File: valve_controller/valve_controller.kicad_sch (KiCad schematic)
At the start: 12 parts, among them J1 CDM1204-04A-FP-F9-67, U1 OPA197xD, U2 ADS1115IDGS, U3 MCP4728, U4 ESP32-S3

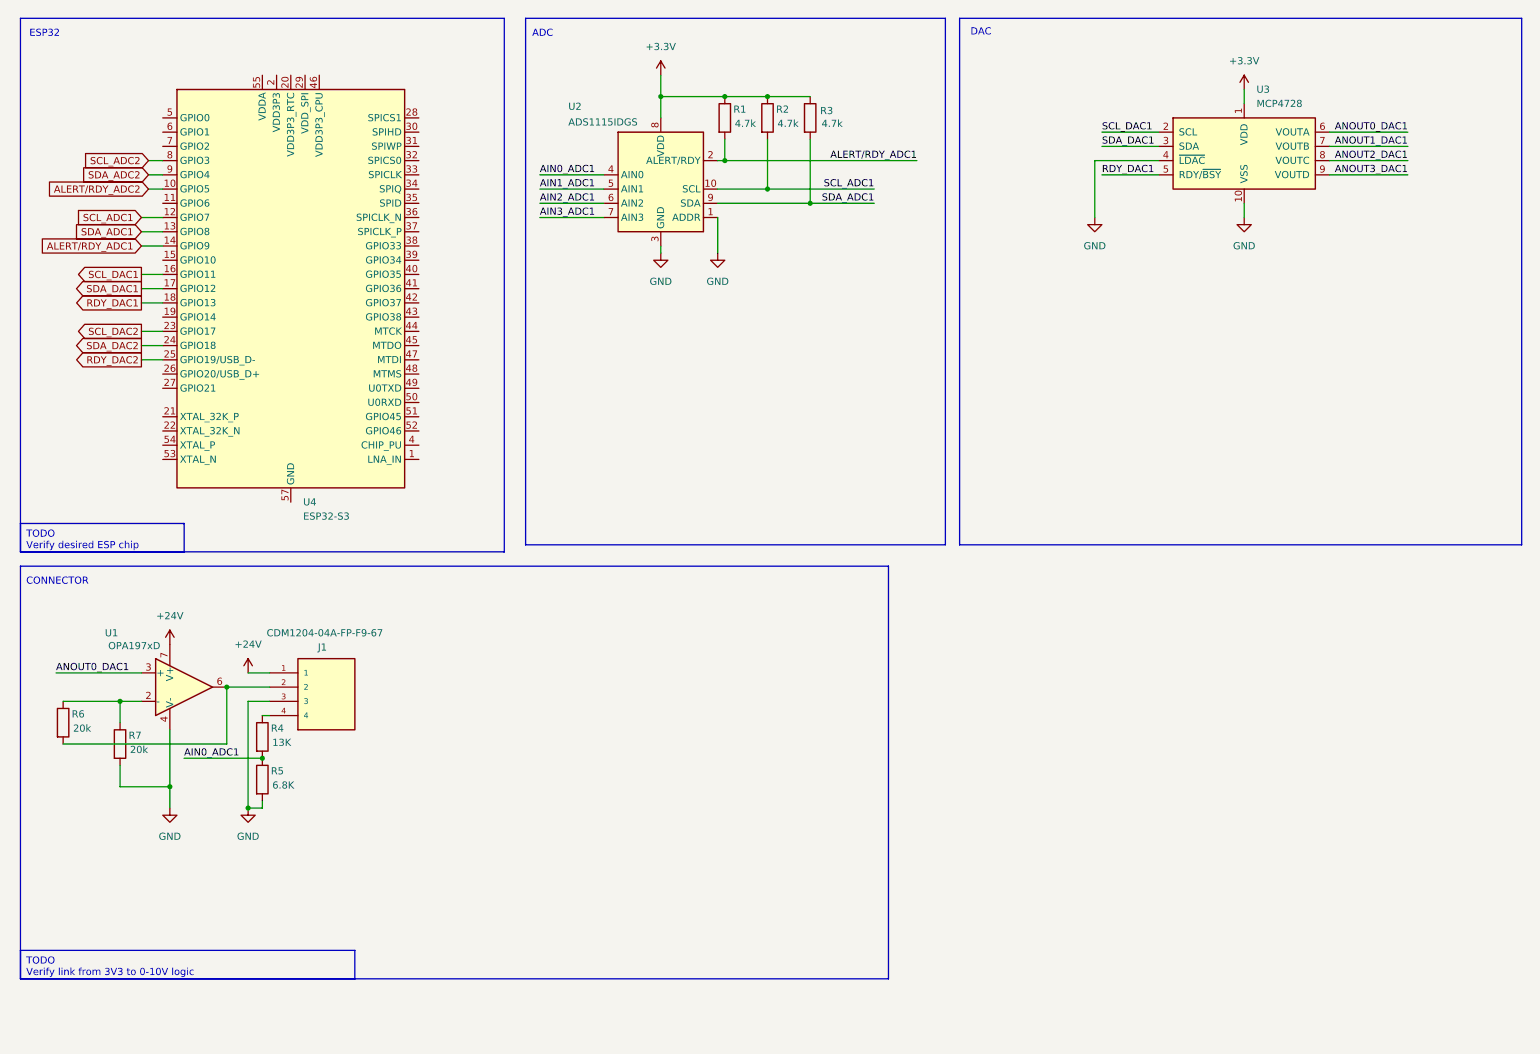
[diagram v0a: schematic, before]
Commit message: First base
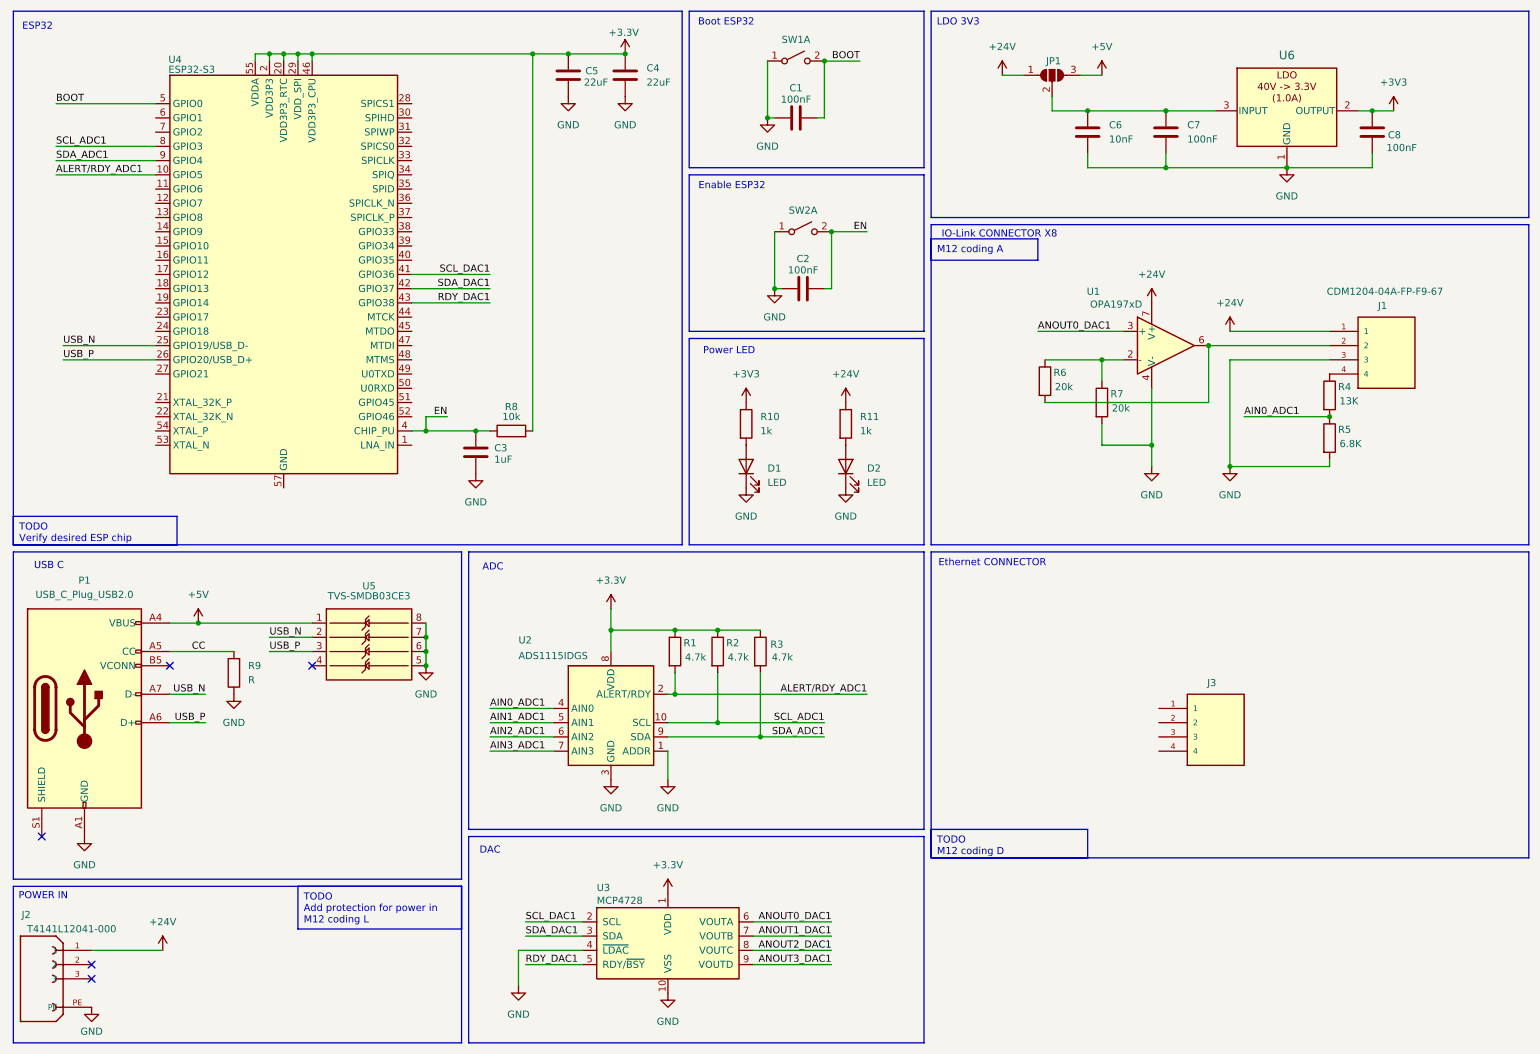
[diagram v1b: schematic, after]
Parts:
- added C1, C2, C7, C8: 100nF, symbol Device:C
- added C3: 1uF, symbol Device:C
- added C4, C5: 22uF, symbol Device:C
- added C6: 10nF, symbol Device:C
- added D1, D2: LED, LED_SMD:LED_0805_2012Metric_Pad1.15x1.40mm_HandSolder, symbol RoverLibrary:LED
- added J2: T4141L12041-000, T4141L12041-000:TE_T4141L12041-000, symbol T4141L12041-000:T4141L12041-000
- added J3: CDM1204-04A-FP-F9-67, CDM1204-04A-FP-F9-67:CUI_CDM1204-04A-FP-F9-67, symbol CDM1204-04A-FP-F9-67:CDM1204-04A-FP-F9-67
- added JP1: SolderJumper_3_Open, symbol Jumper:SolderJumper_3_Open
- added P1: USB_C_Plug_USB2.0, symbol Connector:USB_C_Plug_USB2.0
- added R10, R11: 1k, symbol Device:R
- added R8: 10k, Resistor_SMD:R_0805_2012Metric_Pad1.20x1.40mm_HandSolder, symbol 0_RoverLibrary:R-10k
- added R9: R, symbol Device:R
- added SW1, SW2: SW_DPST_x2, symbol Switch:SW_DPST_x2
- added U5: TVS-SMDB03CE3, Package_SO:SOIC-8_3.9x4.9mm_P1.27mm, symbol RoverLibrary:TVS-SMDB03CE3/TR7TR-ND
- added U6: LDO-LM7805MPX/NOPB, Package_TO_SOT_SMD:TO-252-2, symbol RoverLibrary:LDO-TLE4284DV33ATMA1
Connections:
- net ALERT/RDY_ADC2 is gone; now on net ALERT/RDY_ADC1: U4.10 (GPIO5)
- net SCL_ADC2 is gone; now on net SCL_ADC1: U4.8 (GPIO3)
- net SDA_ADC2 is gone; now on net SDA_ADC1: U4.9 (GPIO4)
- net +24V: now also J2.1, JP1.1 (A), R11.1
- net +3.3V: now also U4.2 (VDD3P3), U4.20 (VDD3P3_RTC), U4.29 (VDD_SPI), U4.3 (VDD3P3), U4.46 (VDD3P3_CPU), U4.55 (VDDA), U4.56 (VDDA), C4.1, C5.1, R8.2
- net ALERT/RDY_ADC1: no longer U4.14 (GPIO9)
- net GND: now also C1.1, C2.1, C3.2, C4.2, C5.2, C6.2, C7.2, C8.2, D1.1 (K), D2.1 (K), J2.PE, P1.A1 (GND), P1.A12 (GND), P1.B1 (GND), P1.B12 (GND), R9.1, SW1.1 (A), SW2.1 (A), U5.5, U5.6, U5.7, U5.8, U6.1 (GND)
- net RDY_DAC1: now also U4.43 (GPIO38); no longer U4.18 (GPIO13)
- net SCL_ADC1: no longer U4.12 (GPIO7)
- net SCL_DAC1: now also U4.41 (GPIO36); no longer U4.16 (GPIO11)
- net SDA_ADC1: no longer U4.13 (GPIO8)
- net SDA_DAC1: now also U4.42 (GPIO37); no longer U4.17 (GPIO12)
- net USB_P: now reaches U4.26 (GPIO20/USB_D+)
- net USB_P: now also P1.A6 (D+), U5.3
- net EN: now reaches U4.4 (CHIP_PU)
- net EN: now also C2.2, C3.1, R8.1, SW2.2 (B)
- net BOOT: now reaches U4.5 (GPIO0)
- net BOOT: now also C1.2, SW1.2 (B)
- net RDY_DAC2 renamed USB_N
- net USB_N: now also P1.A7 (D-), U5.2
- net SCL_DAC2: no longer names the net of U4.23 (GPIO17)
- net SDA_DAC2: no longer names the net of U4.24 (GPIO18)
- new net: C6.1, C7.1, JP1.2 (C), U6.3 (INPUT)
- new net: D2.2 (A), R11.2
- new net: D1.2 (A), R10.2
- new net +3V3: C8.1, R10.1, U6.2 (OUTPUT)
- new net +5V: JP1.3 (B), P1.A4 (VBUS), P1.A9 (VBUS), P1.B4 (VBUS), P1.B9 (VBUS), U5.1
- new net CC: P1.A5 (CC), R9.2
- no-connect marks 0 -> 5
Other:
- note added: "Boot ESP32"
- note added: "Enable ESP32"
- note added: "Ethernet CONNECTOR"
- note added: "IO-Link CONNECTOR X8"
- note added: "LDO 3V3"
- note added: "POWER IN"
- note added: "Power LED"
- note added: "USB C"
- note removed: "CONNECTOR"
- moved on the sheet: J1, R1, R2, R3, R4, R5, R6, R7, U1, U2, U3, U4
